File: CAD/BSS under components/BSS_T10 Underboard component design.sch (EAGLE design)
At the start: 9 parts, among them IC1 7805DT

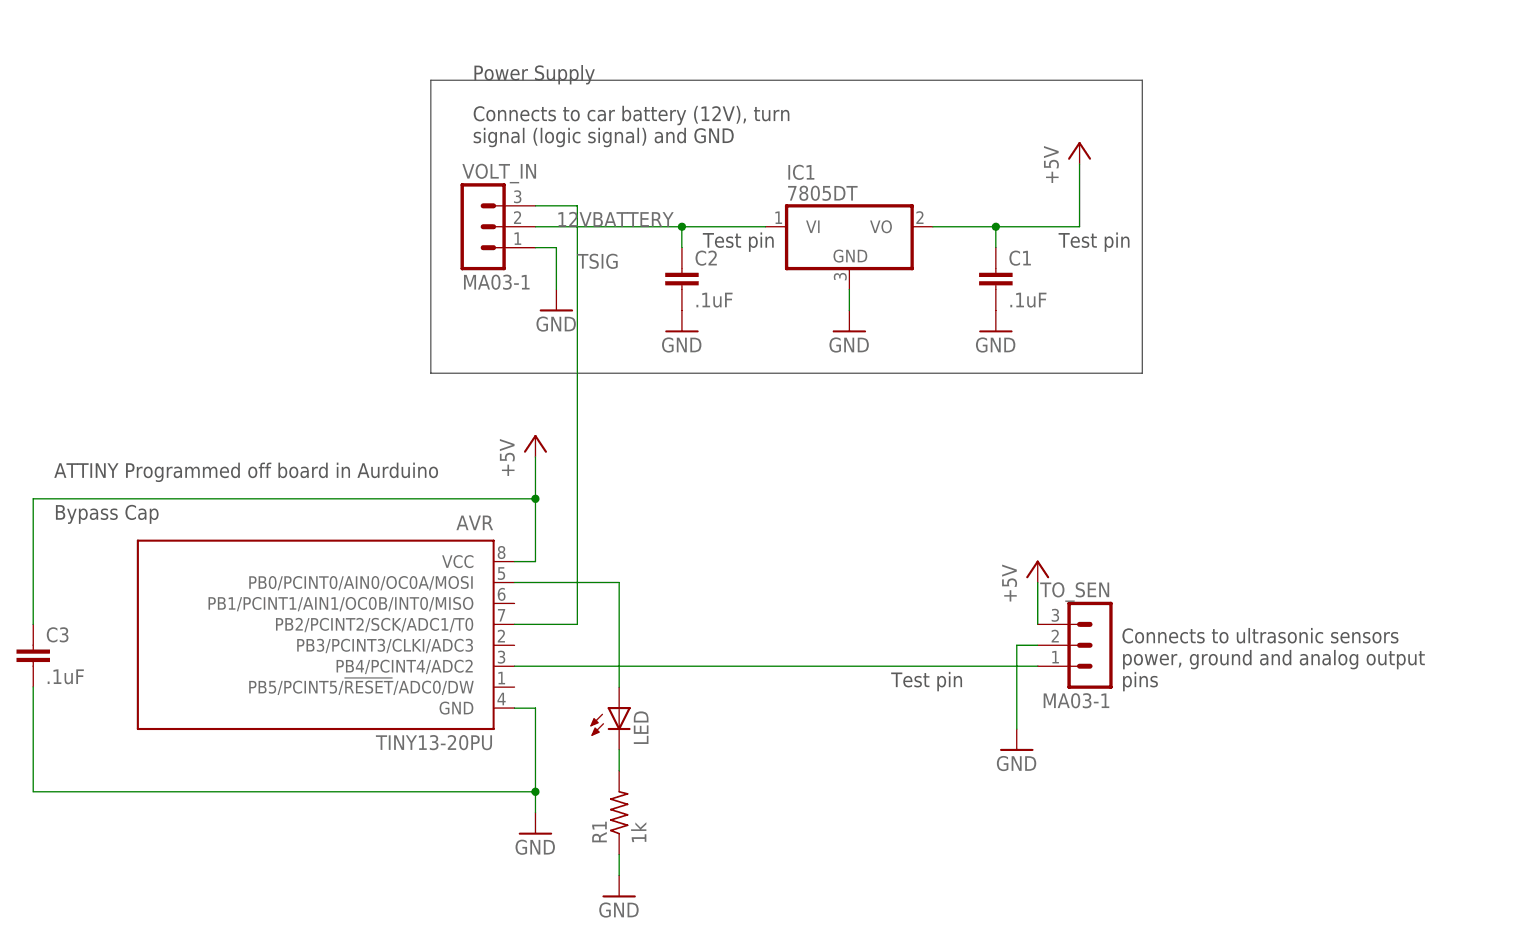
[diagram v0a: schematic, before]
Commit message: New Board Layout
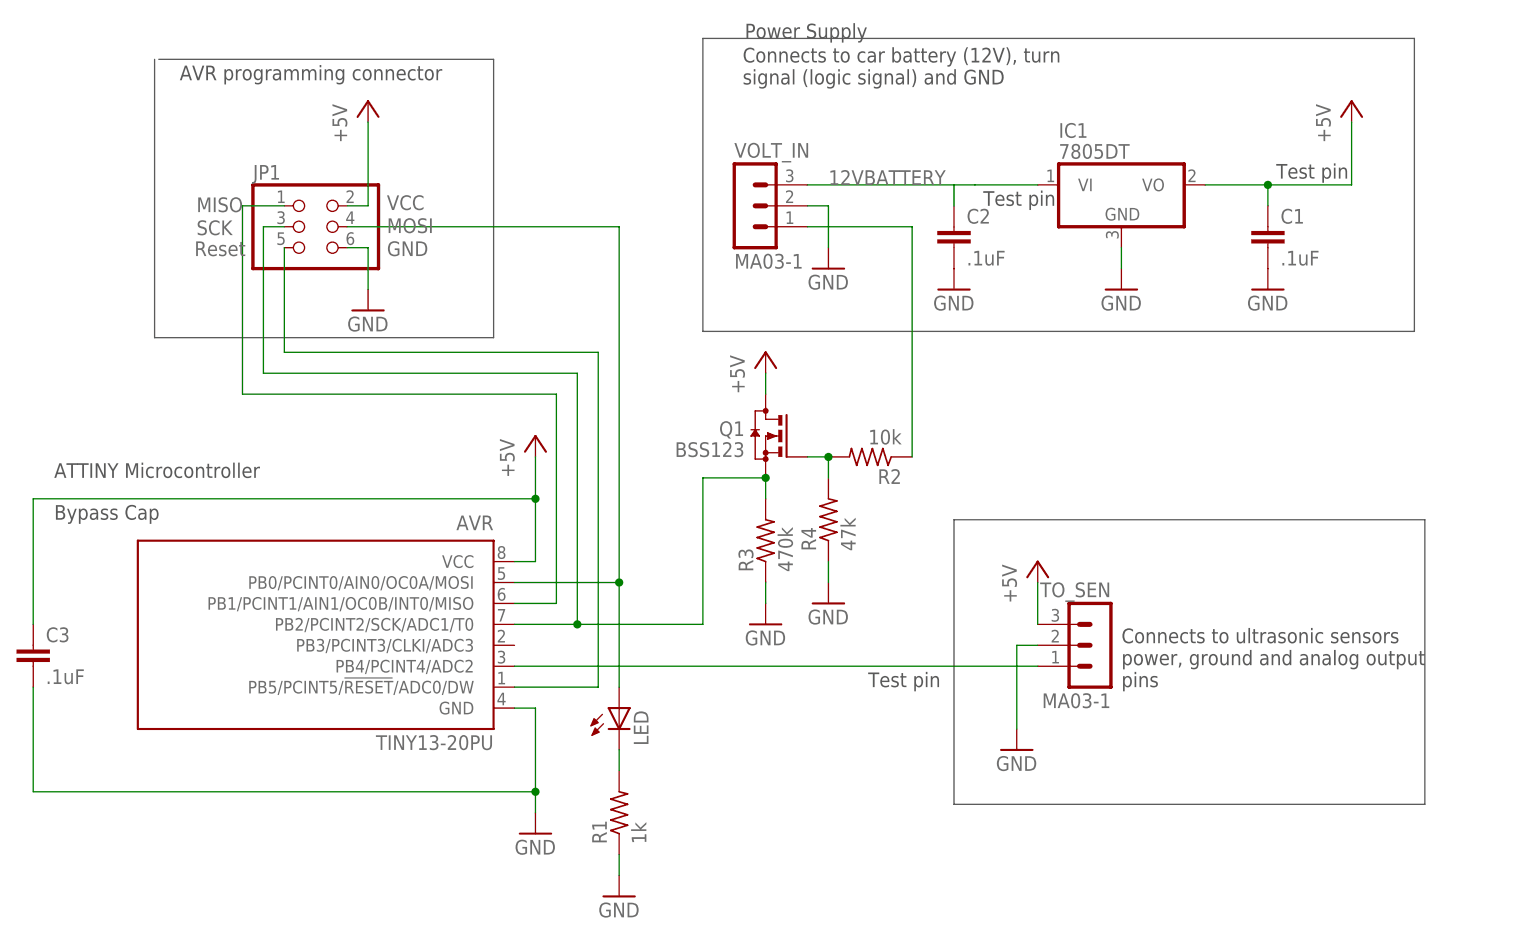
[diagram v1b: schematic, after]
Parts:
- added JP1: (no value), pinhead:PINHD-2X3
- added Q1: BSS123, transistor-small-signal:BSS123
- added R2: 10k, rcl:R-US_R0805
- added R3: 470k, rcl:R-US_R0805
- added R4: 47k, rcl:R-US_R0805
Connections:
- removed net TSIG: AVR.PB2/PCINT2/SCK/ADC1/T0, VOLT_IN.3
- new net 2N7000: AVR.PB2/PCINT2/SCK/ADC1/T0, JP1.3, Q1.S, R3.2
- new net N$5: R2.1, VOLT_IN.1
- new net N$6: Q1.G, R2.2, R4.2
- new net N$7: AVR.PB5/PCINT5/!RESET!/ADC0/DW, JP1.5
- new net N$9: AVR.PB1/PCINT1/AIN1/OC0B/INT0/MISO, JP1.1
- net +5V: now also JP1.2, Q1.D
- net 12VBATTERY: now also VOLT_IN.3; no longer VOLT_IN.2
- net GND: now also JP1.6, R3.1, R4.1, VOLT_IN.2; no longer VOLT_IN.1
- net N$4: now also JP1.4
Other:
- note added: "ATTINY Microcontroller"
- note added: "AVR programming connector"
- note added: "GND"
- note added: "MISO"
- note added: "MOSI"
- note added: "Reset"
- note added: "SCK"
- note added: "VCC"
- note removed: "ATTINY Programmed off board in Aurduino"
- moved on the sheet: C1, C2, IC1, VOLT_IN
